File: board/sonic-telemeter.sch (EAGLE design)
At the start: 24 parts, among them T1 2N2222, T2 2N2222

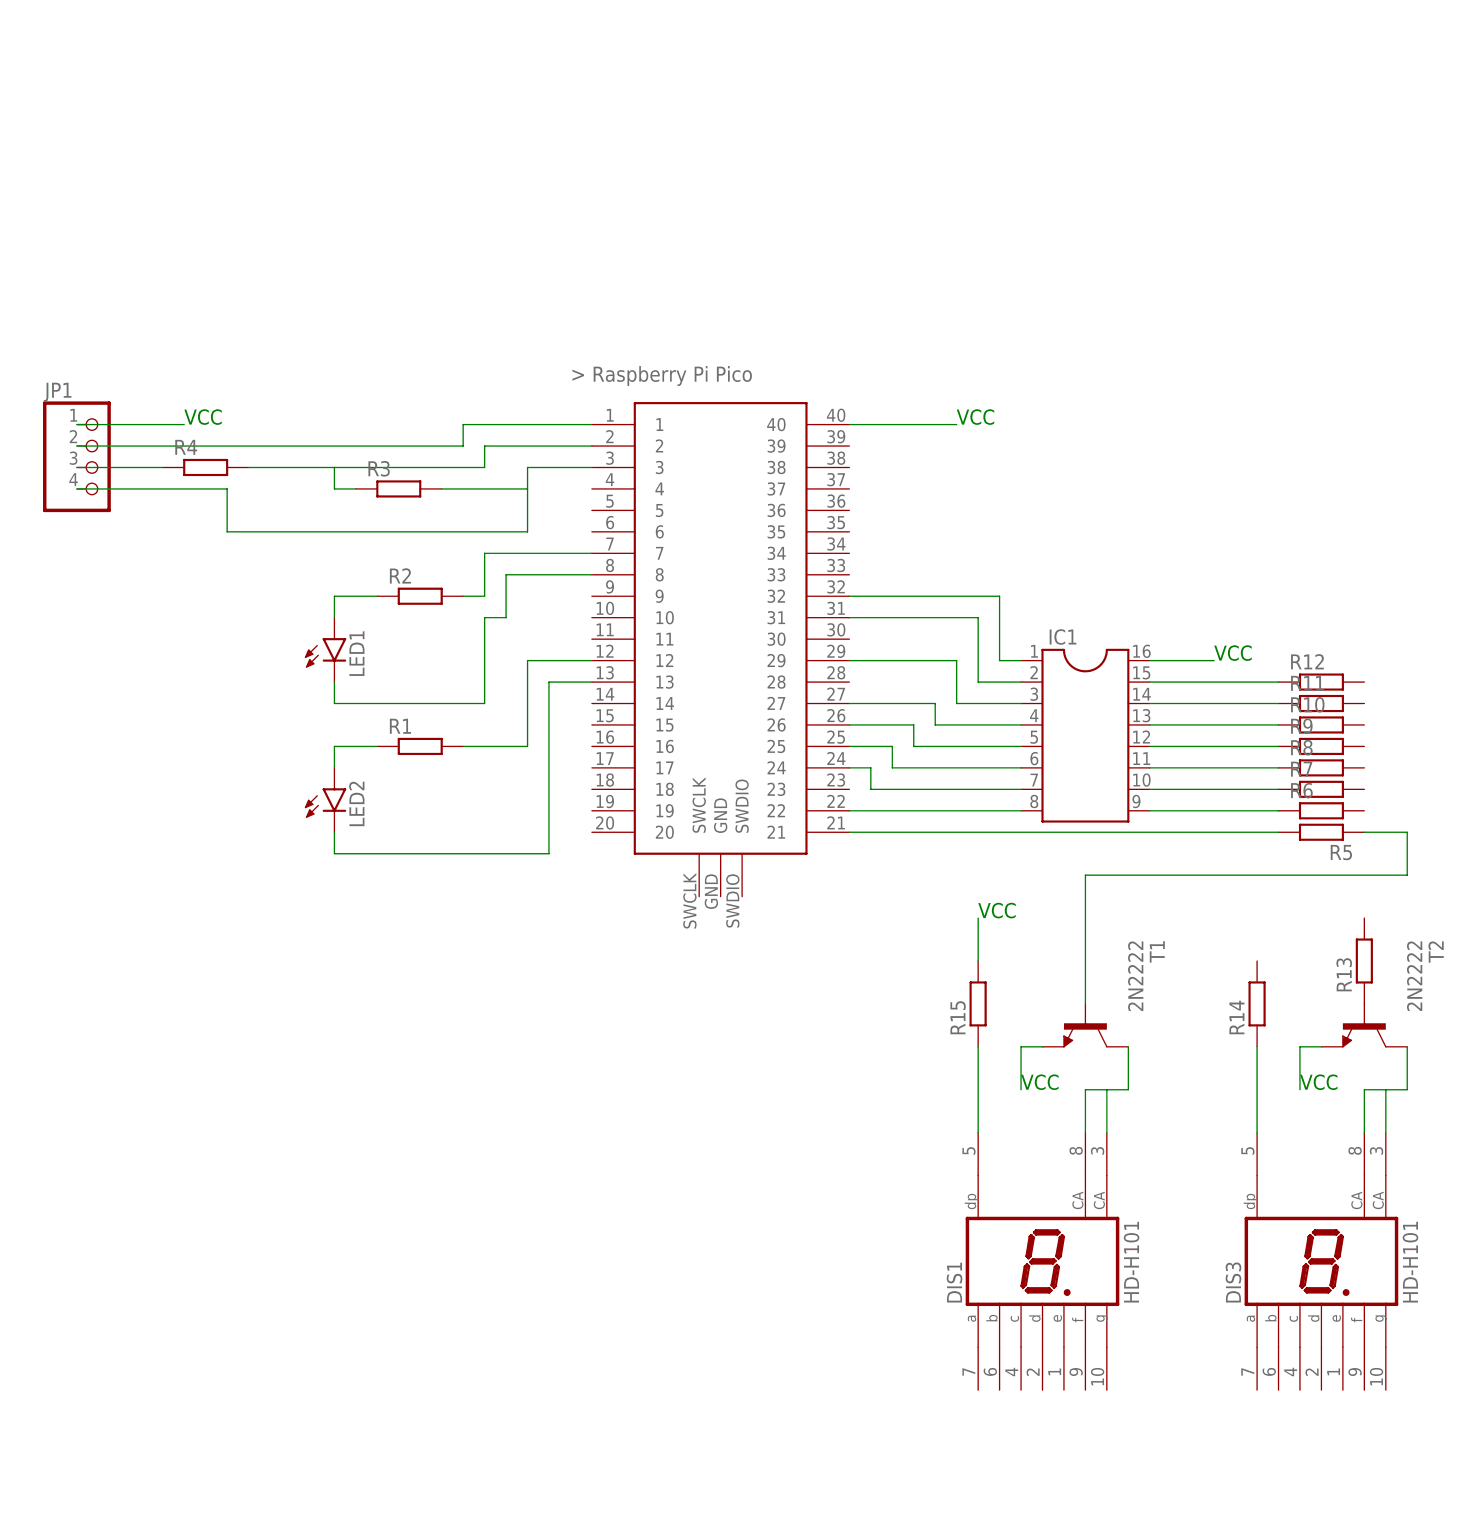
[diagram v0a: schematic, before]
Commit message: Update board schematic
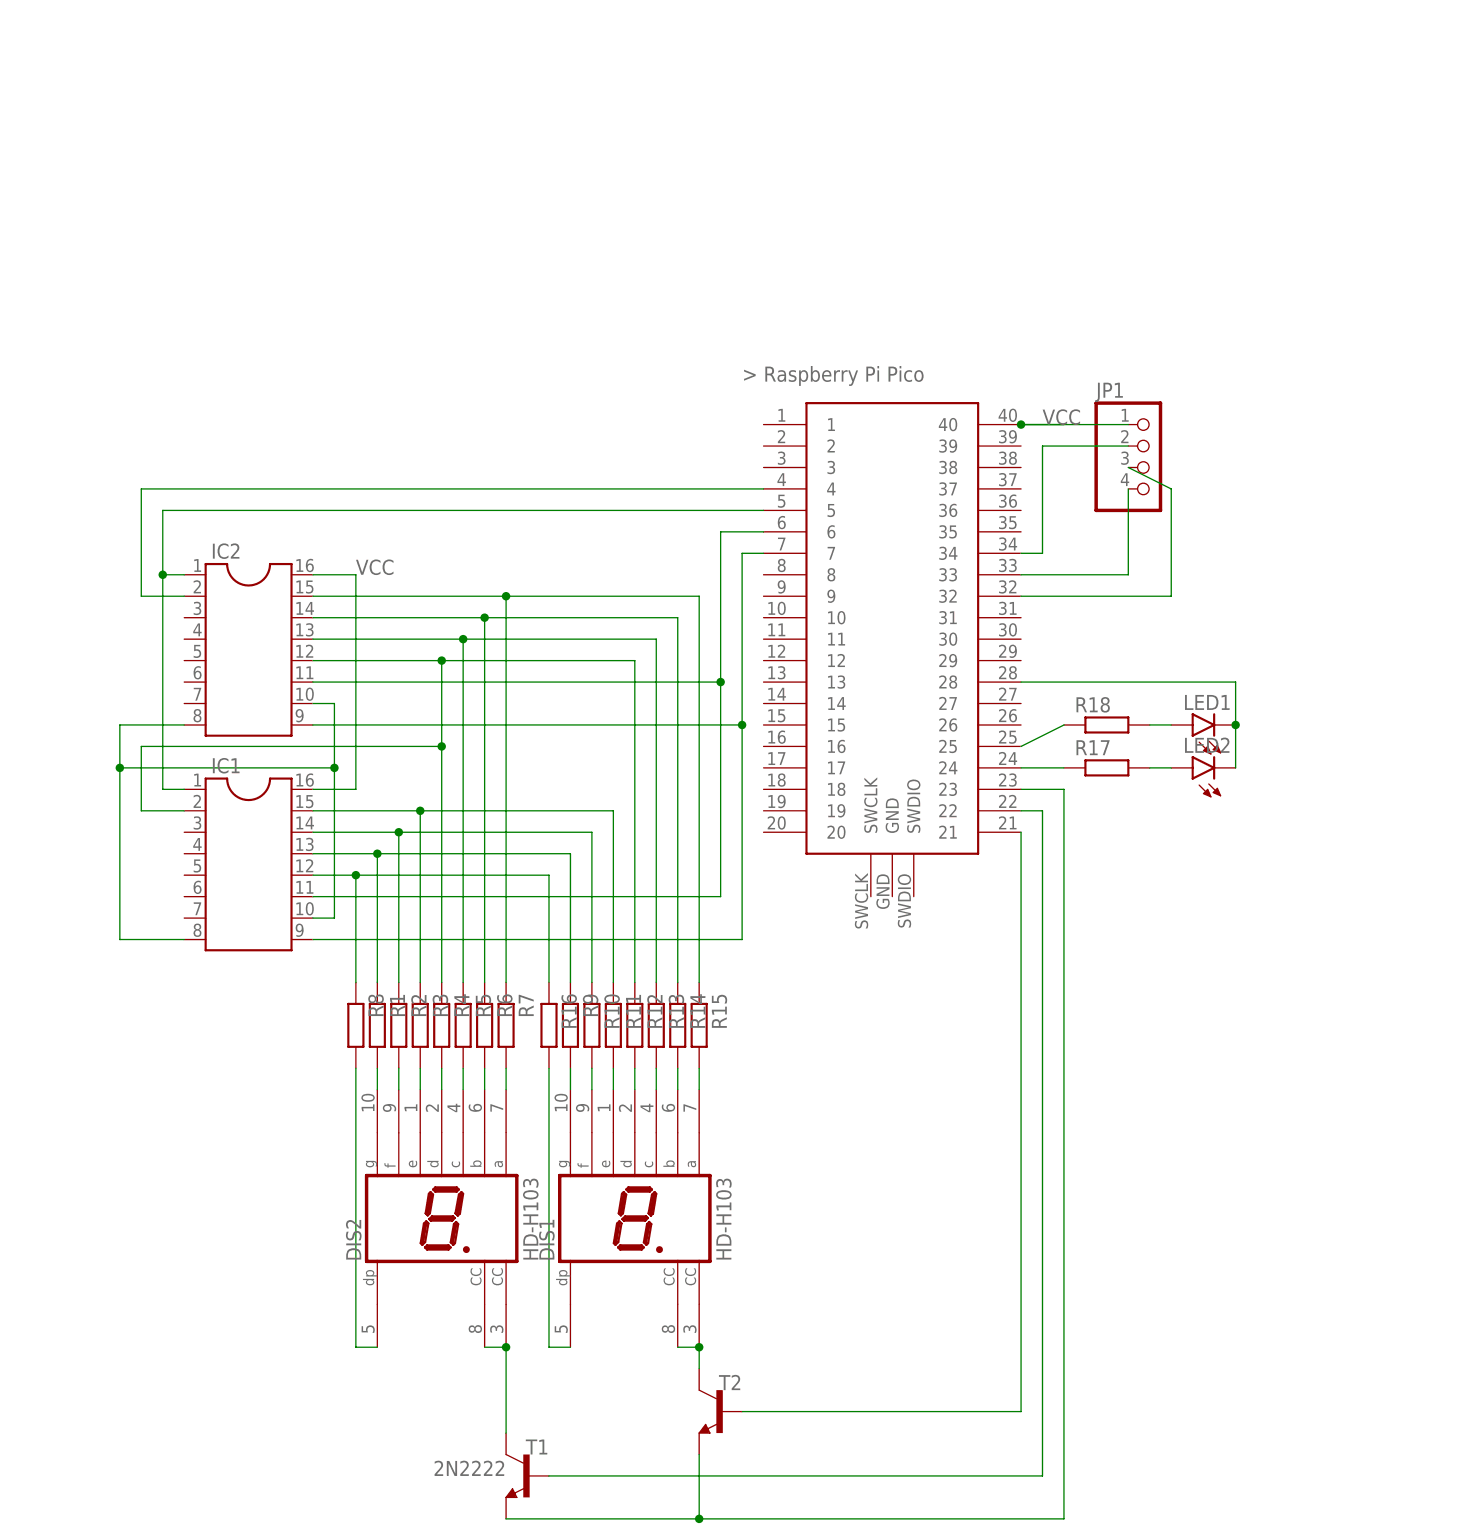
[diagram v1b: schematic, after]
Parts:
- removed DIS3: HD-H101, display-hp:HD-H101
- added DIS2: HD-H103, display-hp:HD-H103
- added IC2: (no value), ic-package:DIL16
- added R16, R17, R18: (no value), rcl:R-EU_0204/5
- DIS1: value HD-H101 -> HD-H103; device display-hp:HD-H101 -> display-hp:HD-H103
- R1, R10, R11, R12, R13, R14, R15, R2, R3, R4, R5, R6, R7, R8, R9: device rcl:R-EU_0204/7 -> rcl:R-EU_0204/5
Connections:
- removed net N$10: LED1.C, U$1.8
- removed net N$37: T1.E
- removed net N$9: JP1.4, R3.2, U$1.3
- new net N$39: T1.B, U$1.22
- new net N$40: R18.1, U$1.25
- new net N$41: R17.1, U$1.24
- new net N$42: LED2.A, R17.2
- new net N$43: LED1.A, R18.2
- new net N$44: LED1.C, LED2.C, U$1.28
- new net N$47: IC1.11, IC2.11, U$1.6
- new net VCC: IC1.16, IC2.16, JP1.1, U$1.40
- net N$1: now also JP1.2, U$1.34; no longer JP1.1
- net N$11: now also IC1.9, IC2.9, U$1.7; no longer R1.2, U$1.12
- net N$12: now also DIS2.G, R1.2; no longer LED2.A, R1.1
- net N$13: now also DIS2.F, R2.2; no longer LED2.C, U$1.13
- net N$14: now also DIS2.E, R3.2; no longer IC1.8, U$1.22
- net N$15: now also DIS2.D, R4.2; no longer IC1.7, U$1.24
- net N$16: now also DIS2.C, R5.2; no longer IC1.6, U$1.25
- net N$17: now also DIS2.B, R6.2; no longer IC1.5, U$1.26
- net N$18: now also DIS2.A, R7.2; no longer IC1.4, U$1.27
- net N$19: now also IC2.12, R12.1, R4.1; no longer U$1.31
- net N$2: now also JP1.4, U$1.33; no longer JP1.2, U$1.1
- net N$20: now also IC2.13, R13.1, R5.1; no longer IC1.3, U$1.29
- net N$21: now also IC2.14, R14.1, R6.1; no longer IC1.1, U$1.32
- net N$22: now also IC2.15, R15.1, R7.1; no longer IC1.15, R12.1
- net N$23: now also DIS2.DP, R8.2; no longer IC1.14, R11.1
- net N$24: now also IC1.15, R11.1, R3.1; no longer IC1.13, R10.1
- net N$25: now also IC1.14, R10.1, R2.1; no longer IC1.12, R9.1
- net N$26: now also IC1.12, R16.1; no longer IC1.11
- net N$27: now also IC1.13, R1.1, R9.1; no longer IC1.10, R7.1
- net N$28: now also DIS1.DP, R16.2; no longer IC1.9, R6.1
- net N$29: now also DIS1.G, R9.2; no longer R5.2, U$1.21
- net N$3: now also U$1.32; no longer R4.1
- net N$30: now also DIS1.F, R10.2; no longer R5.1, T1.B
- net N$31: now also DIS1.E, R11.2; no longer DIS1.CA, DIS1.CA@1, T1.C
- net N$32: now also DIS1.D, R12.2; no longer DIS1.DP, R15.1
- net N$33: now also DIS1.C, R13.2; no longer R15.2
- net N$34: now also DIS1.B, R14.2; no longer DIS3.DP, R14.1
- net N$35: now also DIS1.A, R15.2; no longer DIS3.CA, DIS3.CA@1, T2.C
- net N$36: now also U$1.21; no longer R13.1
- net N$38: now also T1.E, U$1.23
- net N$4: now also IC1.1, IC2.1, U$1.5; no longer R3.1, R4.2, U$1.2
- net N$5: now also IC2.2, U$1.4; no longer R2.2, U$1.7
- net N$6: now also IC1.10, IC1.8, IC2.10, IC2.8; no longer LED1.A, R2.1
- net N$7: now also DIS2.CC, DIS2.CC@1, T1.C; no longer IC1.16
- net N$8: now also DIS1.CC, DIS1.CC@1, T2.C; no longer U$1.40
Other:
- note removed: "VCC"
- moved on the sheet: IC1, JP1, LED1, LED2, R1, R10, R11, R12, R13, R14, R15, R2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

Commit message: Finalize board schematic for intermediary report
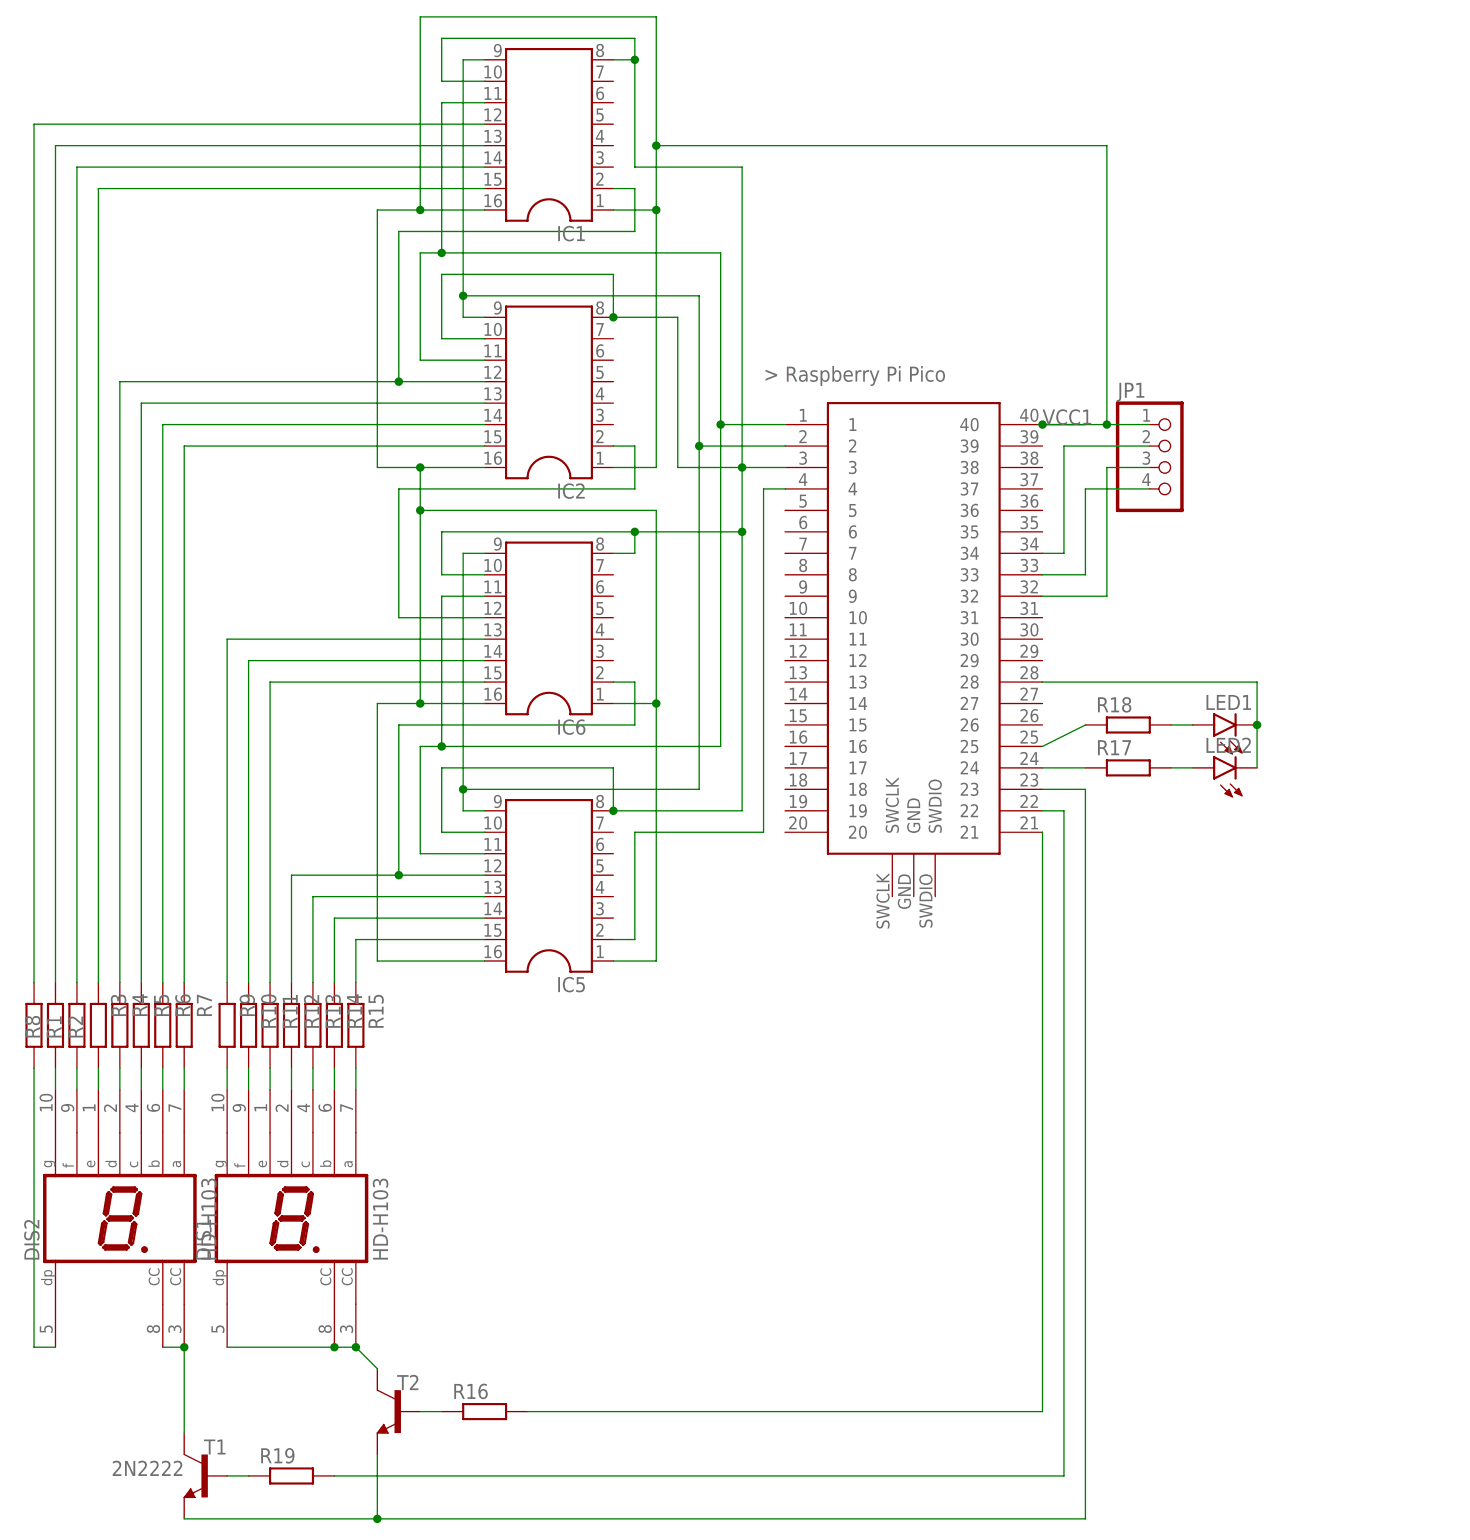
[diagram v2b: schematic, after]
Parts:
- added IC5, IC6: (no value), ic-package:DIL16
- added R19: (no value), rcl:R-EU_0204/5
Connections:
- removed net N$47 (its old number): IC1.11, IC2.11, U$1.6
- removed net VCC: IC1.16, IC2.16, JP1.1, U$1.40
- new net N$10: IC2.13, R5.1
- new net N$2: IC5.2, U$1.4
- new net N$37: IC6.14, R10.1
- new net N$45: IC5.12, IC6.2, R12.1
- new net N$46: IC5.15, R15.1
- new net N$48: IC1.11, IC2.11, IC5.11, IC6.11, U$1.1
- new net N$49: IC1.10, IC1.8, IC2.10, IC2.8, IC5.10, IC5.8, IC6.10, IC6.8, U$1.3
- new net N$51: IC6.15, R11.1
- new net N$9: IC2.14, R6.1
- new net VCC1: IC1.1, IC1.16, IC2.1, IC2.16, IC5.1, IC5.16, IC6.1, IC6.16, JP1.1, U$1.40
- net N$11: now also IC1.2, IC2.12, R4.1; no longer IC1.9, IC2.9, U$1.7
- net N$19: now also IC1.15, R3.1; no longer IC1.2, IC2.12, R12.1, R4.1
- net N$20: now also R16.1, T2.B; no longer IC2.13, R13.1, R5.1
- net N$21: now also IC1.14, R2.1; no longer IC2.14, R14.1, R6.1
- net N$22: now also IC2.2, IC6.12; no longer IC2.15, R15.1, R7.1
- net N$24: now also IC1.13, R1.1; no longer IC1.15, R11.1, R3.1
- net N$25: now also IC1.12, R8.1; no longer IC1.14, R10.1, R2.1
- net N$26: now also IC5.14, R14.1; no longer IC1.12, R16.1, R8.1
- net N$27: now also IC6.13; no longer IC1.13, R1.1
- net N$28: now also R19.1, T1.B; no longer DIS1.DP, R16.2
- net N$36: now also R16.2; no longer T2.B
- net N$39: now also R19.2; no longer T1.B
- net N$4: now also IC1.9, IC2.9, IC5.9, IC6.9, U$1.2; no longer IC1.1, IC2.1, U$1.5
- net N$5: now also IC5.13, R13.1; no longer IC2.2, U$1.4
- net N$6: now also IC2.15, R7.1; no longer IC1.10, IC1.8, IC2.10, IC2.8
- net N$8: now also DIS1.DP
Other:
- moved on the sheet: DIS1, DIS2, IC1, IC2, JP1, LED1, LED2, R1, R10, R11, R12, R13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
